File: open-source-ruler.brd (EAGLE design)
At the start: 86 x 54 mm, 54 parts, among them IC1 LT1007CS8, IC2 FT232RLSSOP, IC3 MDC3105DMT1, IC4 XMEGA16A4A, Q4 ASF1, U1 V_REG_317DPACK, U2 ATMEGA168, U3 ATMEGA168MLF, U4 7432SE, X1 MINI-USB-UX60A-MB-5ST

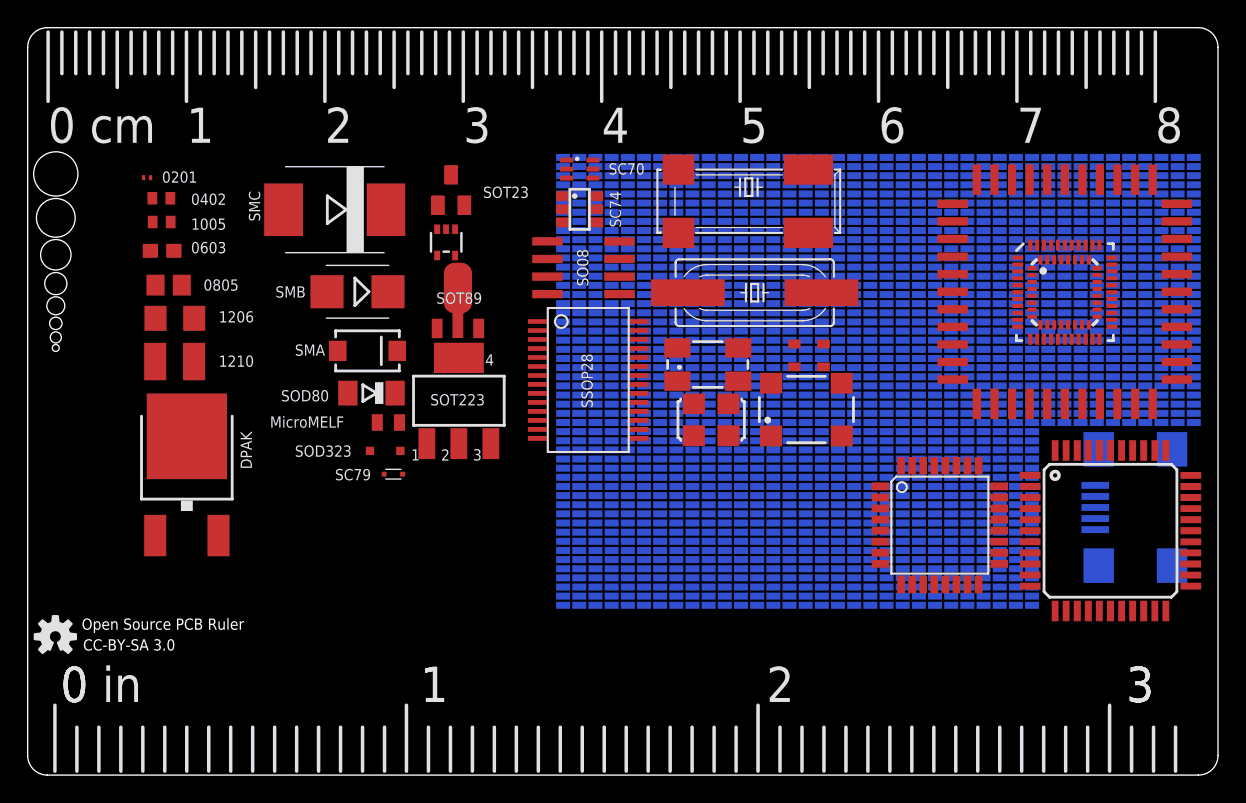
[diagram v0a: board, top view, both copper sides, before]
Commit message: +trace,colour,few FPs
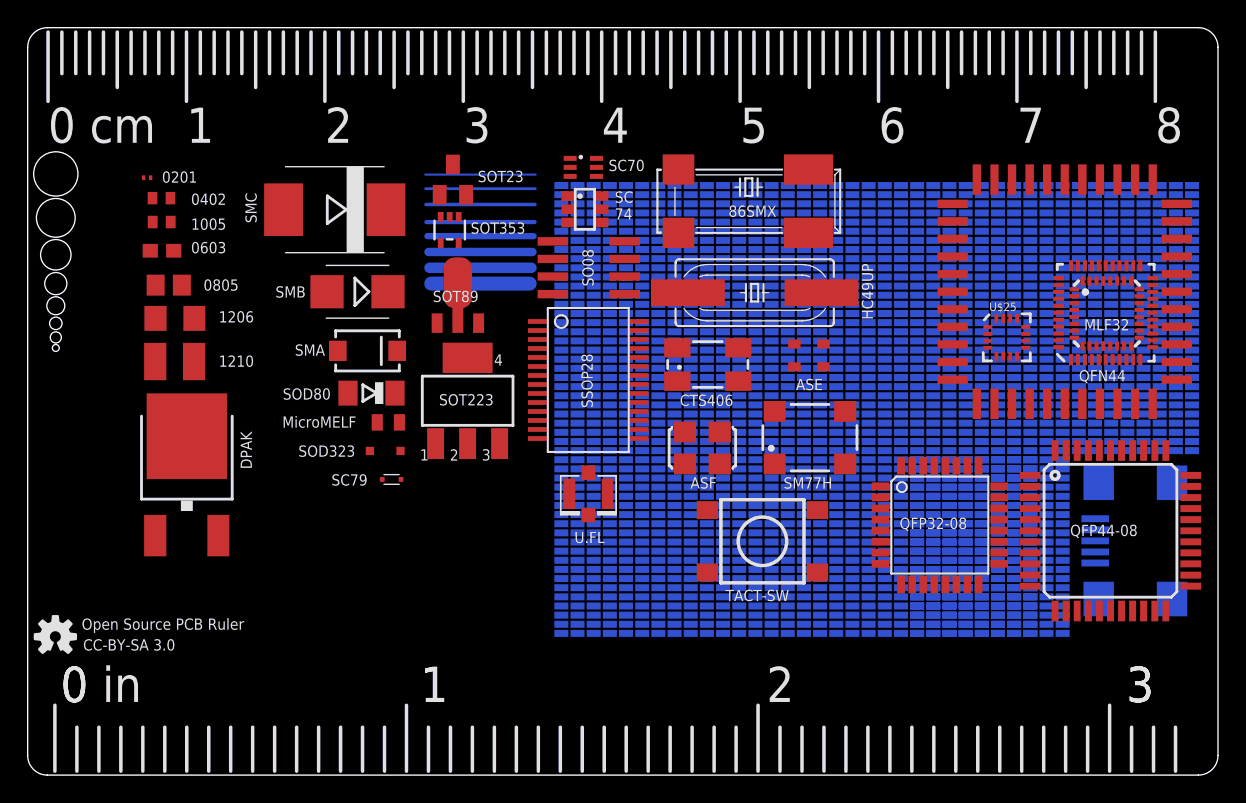
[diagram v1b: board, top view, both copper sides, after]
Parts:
- added S1: SWITCH-MOMENTARY-2, SparkFun:TACTILE_SWITCH_TALL
- added U$23, U$24: PADS, my:PADS
- added U$25: HMC5883LSMD, SparkFun:16LPCC
- added U$26: U.FL, SparkFun:U.FL
- moved U3 3.41 mm to (78.0, 33.4)
- moved U$5 3.30 mm to (77.9, 33.4), turned to 90 degrees
- moved X1 2.41 mm to (79.4, 16.9)
- moved Q4 2.13 mm to (48.7, 23.6)
- moved QG1 2.05 mm to (56.5, 24.4)
- moved U$20 2.04 mm to (43.8, 26.4)
- moved U$21 2.04 mm to (43.8, 19.8)
- moved U$22 2.04 mm to (43.8, 13.2)
- moved U$12 2.04 mm to (67.2, 26.4)
- moved U$13 2.04 mm to (67.2, 19.8)
- moved U$14 2.04 mm to (55.5, 19.8)
- moved U$15 2.04 mm to (55.5, 26.4)
- moved U$4 2.04 mm to (67.2, 13.2)
- moved U$8 2.04 mm to (78.9, 26.4)
- moved U$9 2.04 mm to (55.5, 13.2)
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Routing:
- net N$1: track 0.00 -> 7.98 mm
- net N$2: track 0.00 -> 7.92 mm
- net N$3: track 0.00 -> 7.87 mm
- net N$4: track 0.00 -> 7.82 mm
- net N$5: track 0.00 -> 7.67 mm
- net N$6: track 0.00 -> 7.52 mm
- net N$7: track 0.00 -> 7.37 mm
- net N$8: track 0.00 -> 7.11 mm
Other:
- board text added: "-12"
- board text added: "-3"
- board text added: "-6"
- board text added: "-9"
- board text added: "0 1 2 3 4 5 6 7 8 9"
- board text added: "10"
- board text added: "12"
- board text added: "18"
- board text added: "24"
- board text added: "30"
- board text added: "40"
- board text added: "86SMX"
- board text added: "9"
- board text added: "ASE"
- board text added: "ASF"
- board text added: "CTS406"
- board text added: "Colour Code BLACK BROWN RED ORANGE YELLOW GREEN BLUE VIOLET GRAY WHITE"
- board text added: "GIGA"
- board text added: "HC49UP"
- board text added: "KILO"
- board text added: "MEGA"
- board text added: "MLF32"
- board text added: "PREFIXES"
- board text added: "QFN44"
- board text added: "QFP32-08"
- board text added: "QFP44-08"
- board text added: "SC 74"
- board text added: "SM77H"
- board text added: "SOT353"
- board text added: "TACT-SW"
- board text added: "TERA"
- board text added: "Trace Width(mil)"
- board text added: "U.FL"
- board text added: "micro"
- board text added: "milli"
- board text added: "nano"
- board text added: "pico"
- board text removed: "SC74"
